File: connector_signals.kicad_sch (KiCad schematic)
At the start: 5 parts, among them J1 Conn_01x06, J4 Conn_01x05, J5 Conn_01x05, J6 Conn_01x05, J7 Mega Connector/Breakout (if w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

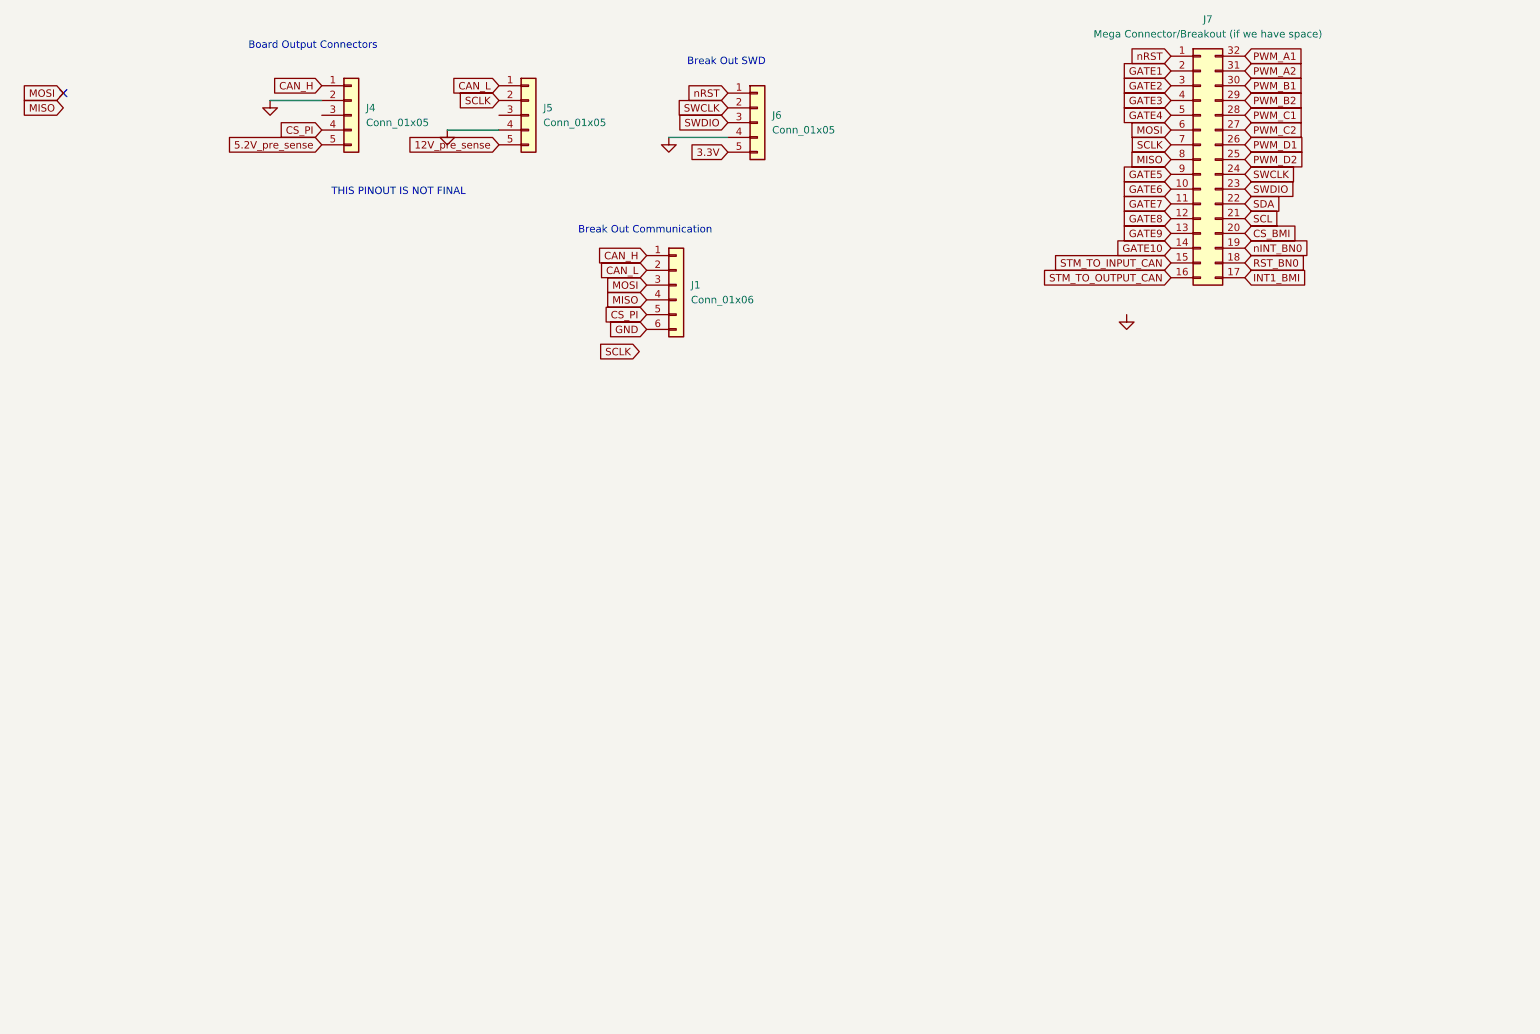
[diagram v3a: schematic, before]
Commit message: We are BACK
I am feeling myself. Lots of progress here.
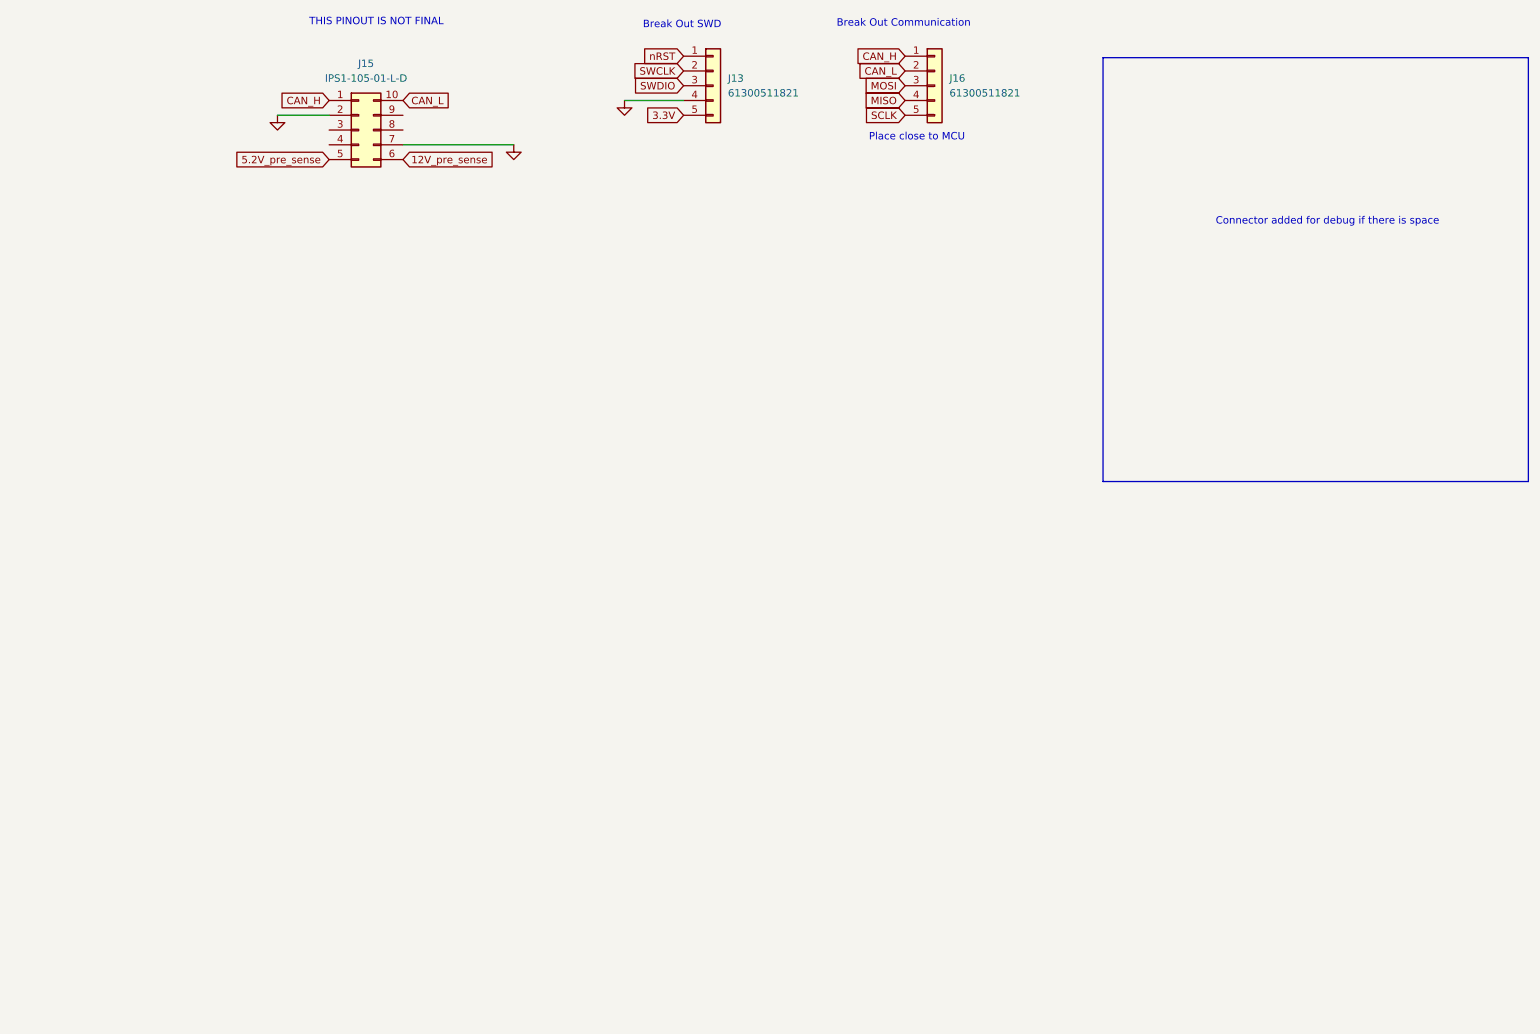
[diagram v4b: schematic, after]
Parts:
- removed J1: Conn_01x06, symbol Connector_Generic:Conn_01x06
- removed J4, J5: Conn_01x05, symbol Connector_Generic:Conn_01x05
- removed J7: Mega Connector/Breakout (if we have space), symbol Connector_Generic:Conn_02x16_Counter_Clockwise
- added J15: IPS1-105-01-L-D, x19_control_library:SAMTEC_IPS1-105-01-S-D, symbol Connector_Generic:Conn_02x05_Counter_Clockwise
- added J16: 61300511821, x19_control_library:61300511821, symbol Connector_Generic:Conn_01x05
- J13: renamed from J6; value Conn_01x05 -> 61300511821; footprint (none) -> x19_control_library:61300511821
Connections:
- net 12V_pre_sense: now also J15.6 (Pin_6)
- net 5.2V_pre_sense: now also J15.5 (Pin_5)
- net CAN_H: now also J15.1 (Pin_1), J16.1 (Pin_1)
- net CAN_L: now also J15.10 (Pin_10), J16.2 (Pin_2)
- net GND: now also J15.2 (Pin_2), J15.7 (Pin_7)
- net MISO: now also J16.4 (Pin_4)
- net MOSI: now also J16.3 (Pin_3)
- net SCLK: now also J16.5 (Pin_5)
- no-connect marks 1 -> 0
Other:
- note added: "Connector added for debug if there is space"
- note added: "Place close to MCU"
- note removed: "Board Output Connectors"
- moved on the sheet: J13
